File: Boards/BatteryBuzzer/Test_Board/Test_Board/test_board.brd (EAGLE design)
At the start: 81.3 x 54.6 mm, 20 parts, among them IC1 ARDUINO_PRO_MICRO

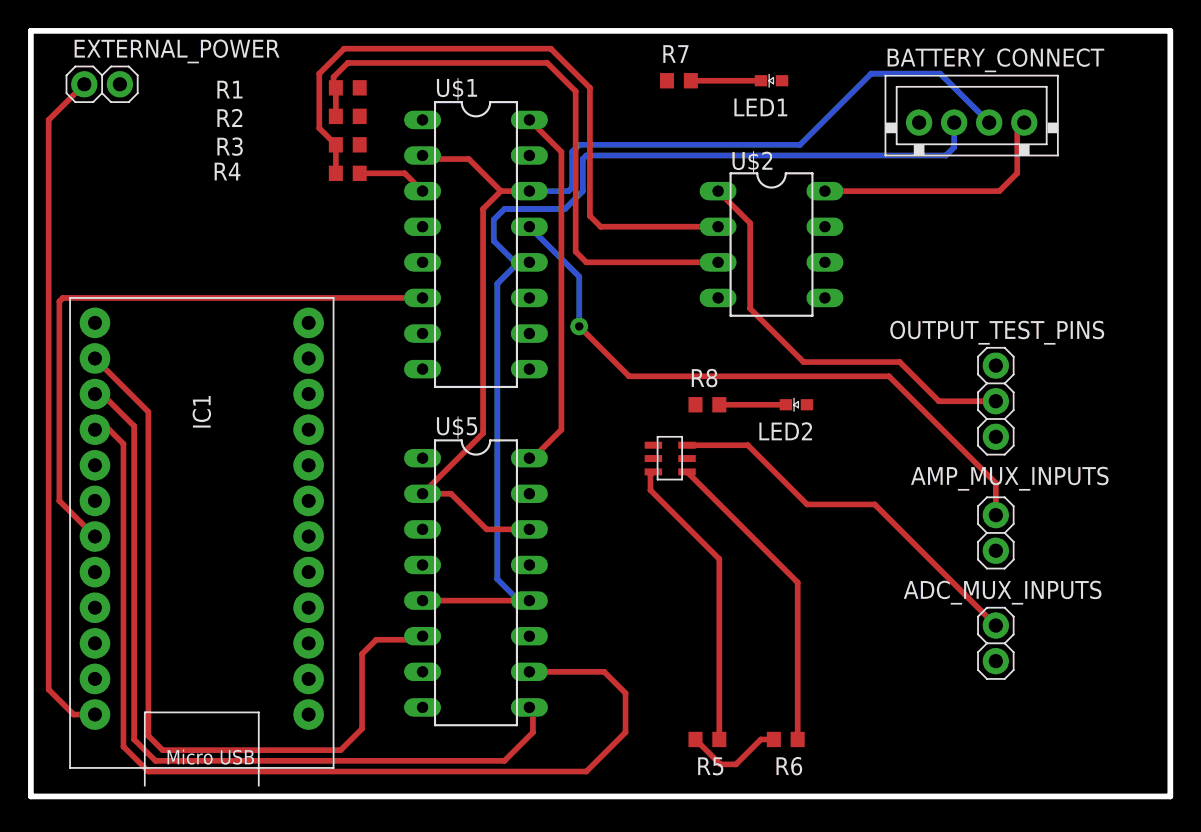
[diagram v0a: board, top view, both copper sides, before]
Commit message: Finished
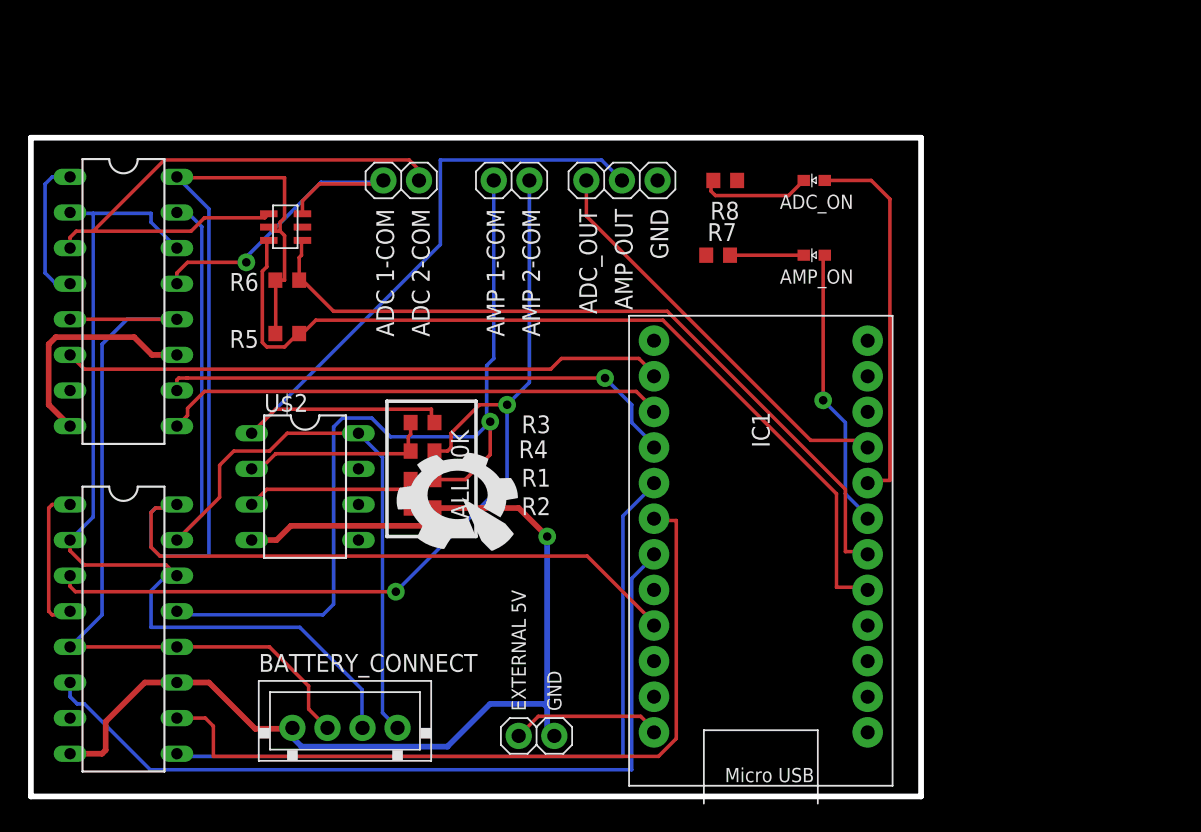
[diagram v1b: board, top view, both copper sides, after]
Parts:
- removed ADC_MUX_INPUTS, AMP_MUX_INPUTS: (no value), pie:1X02
- removed LED1, LED2: GREEN, pie:LED-0603
- removed OUTPUT_TEST_PINS: (no value), pie:1X03
- added ADC_INPUTS, MUX_INPUTS: (no value), pie:1X02
- added ADC_ON, AMP_ON: GREEN, pie:LED-0603
- added OUTPUT: (no value), pie:1X03
- added U$7: (no value), pie:PIE-LOGO-SMALL
- moved BATTERY_CONNECT 62.2 mm to (22.6, 5.08)
- moved EXTERNAL_POWER 55.9 mm to (36.1, 4.32)
- moved R6 48.4 mm to (18.3, 36.8)
- moved R5 41.7 mm to (18.3, 33.0)
- moved IC1 39.9 mm to (61.5, 34.3)
- moved U$2 37.5 mm to (19.6, 22.1)
- moved U$1 37.2 mm to (6.60, 11.9)
- moved U$5 32.2 mm to (6.60, 35.3)
- moved U$3 32.0 mm to (17.3, 42.2)
- moved R2 28.4 mm to (27.9, 20.6)
- moved R1 28.4 mm to (27.9, 22.6)
- moved R4 20.5 mm to (27.9, 24.6)
- moved R3 20.5 mm to (27.9, 26.7)
- moved R8 16.1 mm to (49.5, 43.9), turned to 180 degrees
- moved R7 12.8 mm to (49.0, 38.6)
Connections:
- net 1-COM: now also MUX_INPUTS.2; no longer AMP_MUX_INPUTS.2
- net 2-COM: now also MUX_INPUTS.1; no longer AMP_MUX_INPUTS.1
- net ADC_1-COM: now also ADC_INPUTS.2; no longer ADC_MUX_INPUTS.2
- net ADC_2-COM: now also ADC_INPUTS.1; no longer ADC_MUX_INPUTS.1
- net ADC_OUT: now also OUTPUT.3; no longer OUTPUT_TEST_PINS.3
- net AMP_OUT: now also OUTPUT.2; no longer OUTPUT_TEST_PINS.2
- net GND: now also OUTPUT.1; no longer OUTPUT_TEST_PINS.1
- net LED_1: now also AMP_ON.A; no longer LED1.A
- net LED_2: now also ADC_ON.A; no longer LED2.A
- net N$7: now also ADC_ON.C; no longer LED2.C
- net N$8: now also AMP_ON.C; no longer LED1.C
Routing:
- net GND: track 0.00 -> 116.5 mm, vias 0 -> 1
- net VCC: track 33.2 -> 100.5 mm
- net 2-COM: track 5.01 -> 64.6 mm, vias 0 -> 2
- net A: track 0.00 -> 55.8 mm
- net B: track 0.00 -> 52.3 mm
- net BCELL3: track 18.1 -> 64.9 mm
- net SDA: track 21.2 -> 63.6 mm
- net ADC_2-COM: track 0.00 -> 42.0 mm
- net 5V: track 48.3 -> 10.8 mm
- net ADC_A: track 72.0 -> 37.8 mm, vias 0 -> 1
- net N$3: track 47.4 -> 14.1 mm
- net SCL: track 22.4 -> 54.3 mm
- net N$2: track 43.3 -> 13.8 mm
- net ADC_OUT: track 0.00 -> 29.4 mm
- net LED_2: track 0.00 -> 27.0 mm
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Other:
- board size 81.3 x 54.6 mm -> 63.5 x 47 mm
- board text added: "(c) Pioneers In Engineering Design by: Nick W, Jehan Y This design is open source hardware. For more information, visit: https://github.com/pioneers/PiElectrical"
- board text added: "ADC 1-COM"
- board text added: "ADC 2-COM"
- board text added: "ADC_OUT"
- board text added: "ALL 10K"
- board text added: "AMP 1-COM"
- board text added: "AMP 2-COM"
- board text added: "AMP OUT"
- board text added: "EXTERNAL 5V"
- board text added: "GND"
- board text added: "PIONEERS IN ENGINEERING BATTERY BUZZER SOLUTION TEST BOARD REV 10A"
